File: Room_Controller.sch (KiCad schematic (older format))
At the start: 14 parts, among them P1 Digital, P10 CONN_1, P11 CONN_1, P12 CONN_1, P13 CONN_1, P14 ICSP, P2 Power, P3 Analog, P4 Analog, P5 PWM, P6 PWM, P7 Communication, P8 CONN_1, P9 CONN_1

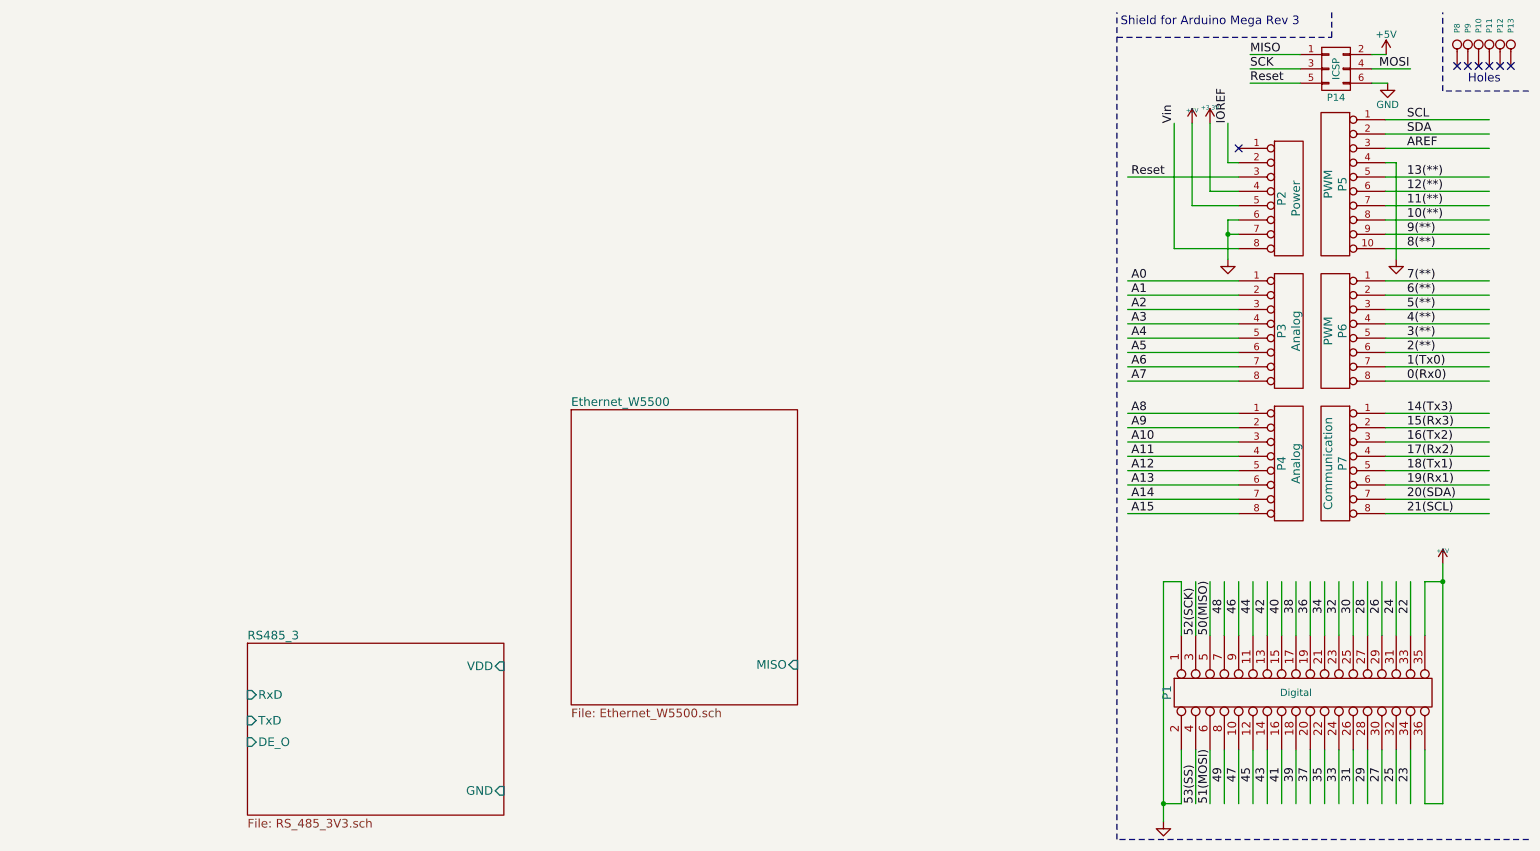
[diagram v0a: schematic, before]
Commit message: Upd
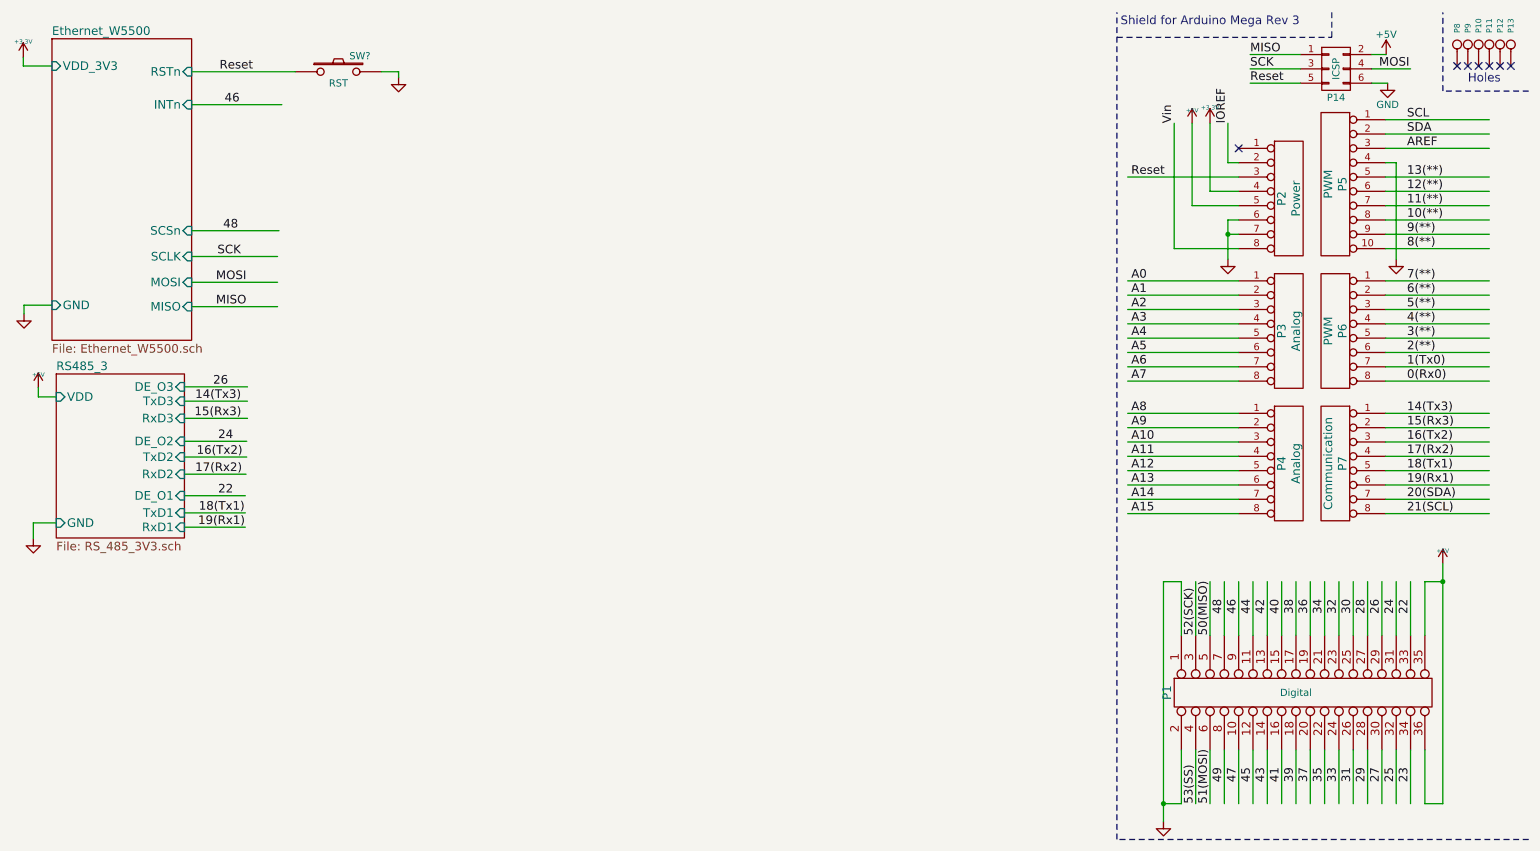
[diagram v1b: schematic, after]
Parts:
- added SW?: RST, BK_Common:SW_SPST_TACT_SMD_3X6, symbol SW_PUSH
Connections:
- wire segments 103 -> 128
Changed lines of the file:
@@
 LIBS:BK_STM8
 LIBS:BK_Common
+LIBS:HR911105A
 LIBS:Room_Controller-cache
 EELAYER 25 0
@@
 AREF
 $Comp
-L +5V #PWR3
+L +5V #PWR01
 U 1 1 5519CA9C
 P 8875 1250
-F 0 "#PWR3" H 8875 1340 20  0001 C CNN
+F 0 "#PWR01" H 8875 1340 20  0001 C CNN
 F 1 "+5V" H 8875 1340 30  0000 C CNN
 F 2 "" H 8875 1250 60  0000 C CNN
@@
 $EndComp
 $Comp
-L +3.3V #PWR4
+L +3.3V #PWR02
 U 1 1 5519CAB8
 P 9000 1250
-F 0 "#PWR4" H 9000 1210 30  0001 C CNN
+F 0 "#PWR02" H 9000 1210 30  0001 C CNN
 F 1 "+3.3V" H 9000 1360 30  0000 C CNN
 F 2 "" H 9000 1250 60  0000 C CNN
@@
 $EndComp
 $Comp
-L GND #PWR6
+L GND #PWR03
 U 1 1 5519CC01
 P 10300 2200
-F 0 "#PWR6" H 10300 2200 30  0001 C CNN
+F 0 "#PWR03" H 10300 2200 30  0001 C CNN
 F 1 "GND" H 10300 2130 30  0001 C CNN
 F 2 "" H 10300 2200 60  0000 C CNN
@@
 $EndComp
 $Comp
-L GND #PWR8
+L GND #PWR04
 U 1 1 5519CDF8
 P 8675 6125
-F 0 "#PWR8" H 8675 6125 30  0001 C CNN
+F 0 "#PWR04" H 8675 6125 30  0001 C CNN
 F 1 "GND" H 8675 6055 30  0001 C CNN
 F 2 "" H 8675 6125 60  0000 C CNN
@@
 $EndComp
 $Comp
-L +5V #PWR7
+L +5V #PWR05
 U 1 1 5519D165
 P 10625 4325
-F 0 "#PWR7" H 10625 4415 20  0001 C CNN
+F 0 "#PWR05" H 10625 4415 20  0001 C CNN
 F 1 "+5V" H 10625 4415 30  0000 C CNN
 F 2 "" H 10625 4325 60  0000 C CNN
@@
 Holes
 $Comp
-L GND #PWR5
+L GND #PWR06
 U 1 1 5519C84C
 P 9125 2200
-F 0 "#PWR5" H 9125 2200 30  0001 C CNN
+F 0 "#PWR06" H 9125 2200 30  0001 C CNN
 F 1 "GND" H 9125 2130 30  0001 C CNN
 F 2 "" H 9125 2200 60  0000 C CNN
@@
 	1    0    0    -1
 $EndComp
+$Comp
+L CONN_02X03 P14
+U 1 1 56F8AE8E
+P 9880 870
+F 0 "P14" H 9880 670 50  0000 C CNN
+F 1 "ICSP" V 9880 870 50  0000 C CNN
+F 2 "Pin_Headers:Pin_Header_Straight_2x03" H 9880 -330 50  0001 C CNN
+F 3 "" H 9880 -330 50  0000 C CNN
+	1    9880 870
+	1    0    0    -1
+$EndComp
+Text Label 9280 770  0    60   ~ 0
+MISO
+$Comp
+L +5V #PWR07
+U 1 1 56F8B737
+P 10230 770
+F 0 "#PWR07" H 10230 620 50  0001 C CNN
+F 1 "+5V" H 10230 910 50  0000 C CNN
+F 2 "" H 10230 770 50  0000 C CNN
+F 3 "" H 10230 770 50  0000 C CNN
+	1    10230 770
+	1    0    0    -1
+$EndComp
+Text Label 9280 870  0    60   ~ 0
+SCK
+Text Label 9280 970  0    60   ~ 0
+Reset
+Text Label 10180 870  0    60   ~ 0
+MOSI
+$Comp
+L GND #PWR08
+U 1 1 56F8B93D
+P 10240 970
+F 0 "#PWR08" H 10240 720 50  0001 C CNN
+F 1 "GND" H 10240 820 50  0000 C CNN
+F 2 "" H 10240 970 50  0000 C CNN
+F 3 "" H 10240 970 50  0000 C CNN
+	1    10240 970
+	1    0    0    -1
+$EndComp
+$Sheet
+S 915  660  975  2105
+U 56F8E6BF
+F0 "Ethernet_W5500" 60
+F1 "Ethernet_W5500.sch" 60
+F2 "MISO" I R 1890 2530 60
+F3 "MOSI" I R 1890 2360 60
+F4 "SCSn" I R 1890 2000 60
+F5 "SCLK" I R 1890 2180 60
+F6 "INTn" I R 1890 1120 60
+F7 "RSTn" I R 1890 890 60
+F8 "VDD_3V3" I L 915 850 60
+F9 "GND" I L 915 2520 60
+$EndSheet
+$Comp
+L +3.3V #PWR09
+U 1 1 56FCFCED
+P 715 790
+F 0 "#PWR09" H 715 750 30  0001 C CNN
+F 1 "+3.3V" H 715 900 30  0000 C CNN
+F 2 "" H 715 790 60  0000 C CNN
+F 3 "" H 715 790 60  0000 C CNN
+	1    715  790
+	1    0    0    -1
+$EndComp
+$Comp
+L GND #PWR010
+U 1 1 56FD0674
+P 720 2580
+F 0 "#PWR010" H 720 2580 30  0001 C CNN
+F 1 "GND" H 720 2510 30  0001 C CNN
+F 2 "" H 720 2580 60  0000 C CNN
+F 3 "" H 720 2580 60  0000 C CNN
+	1    720  2580
+	1    0    0    -1
+$EndComp
+$Comp
+L GND #PWR011
+U 1 1 56FD647A
+P 785 4150
+F 0 "#PWR011" H 785 4150 30  0001 C CNN
+F 1 "GND" H 785 4080 30  0001 C CNN
+F 2 "" H 785 4150 60  0000 C CNN
+F 3 "" H 785 4150 60  0000 C CNN
+	1    785  4150
+	1    0    0    -1
+$EndComp
+$Comp
+L +5V #PWR012
+U 1 1 56FD66CB
+P 820 3095
+F 0 "#PWR012" H 820 3185 20  0001 C CNN
+F 1 "+5V" H 820 3185 30  0000 C CNN
+F 2 "" H 820 3095 60  0000 C CNN
+F 3 "" H 820 3095 60  0000 C CNN
+	1    820  3095
+	1    0    0    -1
+$EndComp
+Text Label 1935 4070 0    60   ~ 0
+19(Rx1)
+Text Label 1940 3970 0    60   ~ 0
+18(Tx1)
+Text Label 1915 3700 0    60   ~ 0
+17(Rx2)
+Text Label 1925 3580 0    60   ~ 0
+16(Tx2)
+Text Label 1910 3310 0    60   ~ 0
+15(Rx3)
+Text Label 1915 3190 0    60   ~ 0
+14(Tx3)
+Text Label 2180 3850 2    60   ~ 0
+22
+Text Label 2180 3470 2    60   ~ 0
+24
+Text Label 2145 3090 2    60   ~ 0
+26
 Wire Wire Line
 	8900 4450 8900 4825
@@
 	10225 2125 10950 2125
 Wire Wire Line
-	9125 2200 9125 1925
+	9125 1925 9125 2200
 Wire Wire Line
 	9125 1925 9200 1925
@@
 Wire Wire Line
 	10300 1525 10225 1525
-$Comp
-L CONN_02X03 P14
-U 1 1 56F8AE8E
-P 9880 870
-F 0 "P14" H 9880 670 50  0000 C CNN
-F 1 "ICSP" V 9880 870 50  0000 C CNN
-F 2 "Pin_Headers:Pin_Header_Straight_2x03" H 9880 -330 50  0001 C CNN
-F 3 "" H 9880 -330 50  0000 C CNN
-	1    9880 870
-	1    0    0    -1
-$EndComp
 Wire Wire Line
 	9630 770  9280 770
@@
 Wire Wire Line
 	9630 970  9280 970
-Text Label 9280 770  0    60   ~ 0
+Wire Wire Line
+	10130 770  10230 770
+Wire Wire Line
+	10130 970  10240 970
+Wire Wire Line
+	10130 870  10400 870
+Wire Wire Line
+	720  2580 720  2520
+Wire Wire Line
+	720  2520 915  2520
+Wire Wire Line
+	715  790  715  850
+Wire Wire Line
+	715  850  915  850
+Wire Wire Line
+	820  3095 820  3160
+Wire Wire Line
+	820  3160 945  3160
+Wire Wire Line
+	785  4150 785  4040
+Wire Wire Line
+	785  4040 945  4040
+Wire Wire Line
+	1840 4070 2265 4070
+Wire Wire Line
+	1840 3970 2265 3970
+Wire Wire Line
+	1840 3850 2265 3850
+Wire Wire Line
+	1840 3700 2270 3700
+Wire Wire Line
+	1840 3580 2275 3580
+Wire Wire Line
+	1840 3470 2275 3470
+Wire Wire Line
+	1840 3310 2280 3310
+Wire Wire Line
+	1840 3190 2280 3190
+Wire Wire Line
+	1840 3090 2280 3090
+Wire Wire Line
+	1890 2530 2490 2530
+Wire Wire Line
+	1890 2360 2490 2360
+Wire Wire Line
+	1890 2180 2490 2180
+Wire Wire Line
+	1890 2000 2500 2000
+Wire Wire Line
+	1890 890  2615 890
+Wire Wire Line
+	1890 1120 2520 1120
+Text Label 2215 2000 2    60   ~ 0
+48
+Text Label 2070 2180 0    60   ~ 0
+SCK
+Text Label 2060 2360 0    60   ~ 0
+MOSI
+Text Label 2060 2530 0    60   ~ 0
 MISO
-$Comp
-L +5V #PWR1
-U 1 1 56F8B737
-P 10230 770
-F 0 "#PWR1" H 10230 620 50  0001 C CNN
-F 1 "+5V" H 10230 910 50  0000 C CNN
-F 2 "" H 10230 770 50  0000 C CNN
-F 3 "" H 10230 770 50  0000 C CNN
-	1    10230 770
-	1    0    0    -1
-$EndComp
-Wire Wire Line
-	10130 770  10230 770
-Text Label 9280 870  0    60   ~ 0
-SCK
-Text Label 9280 970  0    60   ~ 0
+Text Label 2225 1120 2    60   ~ 0
+46
+Text Label 2085 890  0    60   ~ 0
 Reset
-Text Label 10180 870  0    60   ~ 0
-MOSI
-$Comp
-L GND #PWR2
-U 1 1 56F8B93D
-P 10240 970
-F 0 "#PWR2" H 10240 720 50  0001 C CNN
-F 1 "GND" H 10240 820 50  0000 C CNN
-F 2 "" H 10240 970 50  0000 C CNN
-F 3 "" H 10240 970 50  0000 C CNN
-	1    10240 970
-	1    0    0    -1
-$EndComp
-Wire Wire Line
-	10130 970  10240 970
-Wire Wire Line
-	10130 870  10400 870
 $Sheet
-S 4540 3250 1580 2060
-U 56F8E6BF
-F0 "Ethernet_W5500" 60
-F1 "Ethernet_W5500.sch" 60
-F2 "MISO" I R 6120 5030 60
-$EndSheet
-$Sheet
-S 2280 4880 1790 1200
+S 945  3000 895  1145
 U 56F8BFFB
 F0 "RS485_3" 60
 F1 "RS_485_3V3.sch" 60
-F2 "GND" I R 4070 5910 60
-F3 "VDD" I R 4070 5040 60
-F4 "RxD" I L 2280 5240 60
-F5 "TxD" I L 2280 5420 60
-F6 "DE_O" I L 2280 5570 60
+F2 "GND" I L 945 4040 60
+F3 "VDD" I L 945 3160 60
+F4 "RxD1" I R 1840 4070 60
+F5 "TxD1" I R 1840 3970 60
+F6 "DE_O1" I R 1840 3850 60
+F7 "RxD2" I R 1840 3700 60
+F8 "TxD2" I R 1840 3580 60
+F9 "DE_O2" I R 1840 3470 60
+F10 "RxD3" I R 1840 3310 60
+F11 "TxD3" I R 1840 3190 60
+F12 "DE_O3" I R 1840 3090 60
 $EndSheet
+$Comp
+L SW_PUSH SW?
+U 1 1 5700B218
+P 2915 890
+F 0 "SW?" H 3065 1000 50  0000 C CNN
+F 1 "RST" H 2915 810 50  0000 C CNN
+F 2 "BK_Common:SW_SPST_TACT_SMD_3X6" H 2915 890 50  0001 C CNN
+F 3 "" H 2915 890 50  0000 C CNN
+	1    2915 890
+	1    0    0    -1
+$EndComp
+$Comp
+L GND #PWR?
+U 1 1 5700CBCC
+P 3335 930
+F 0 "#PWR?" H 3335 930 30  0001 C CNN
+F 1 "GND" H 3335 860 30  0001 C CNN
+F 2 "" H 3335 930 60  0000 C CNN
+F 3 "" H 3335 930 60  0000 C CNN
+	1    3335 930
+	1    0    0    -1
+$EndComp
+Wire Wire Line
+	3215 890  3335 890
+Wire Wire Line
+	3335 890  3335 930
 $EndSCHEMATC
